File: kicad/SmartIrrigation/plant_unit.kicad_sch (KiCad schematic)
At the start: 10 parts, among them T1 RJ45 Connector

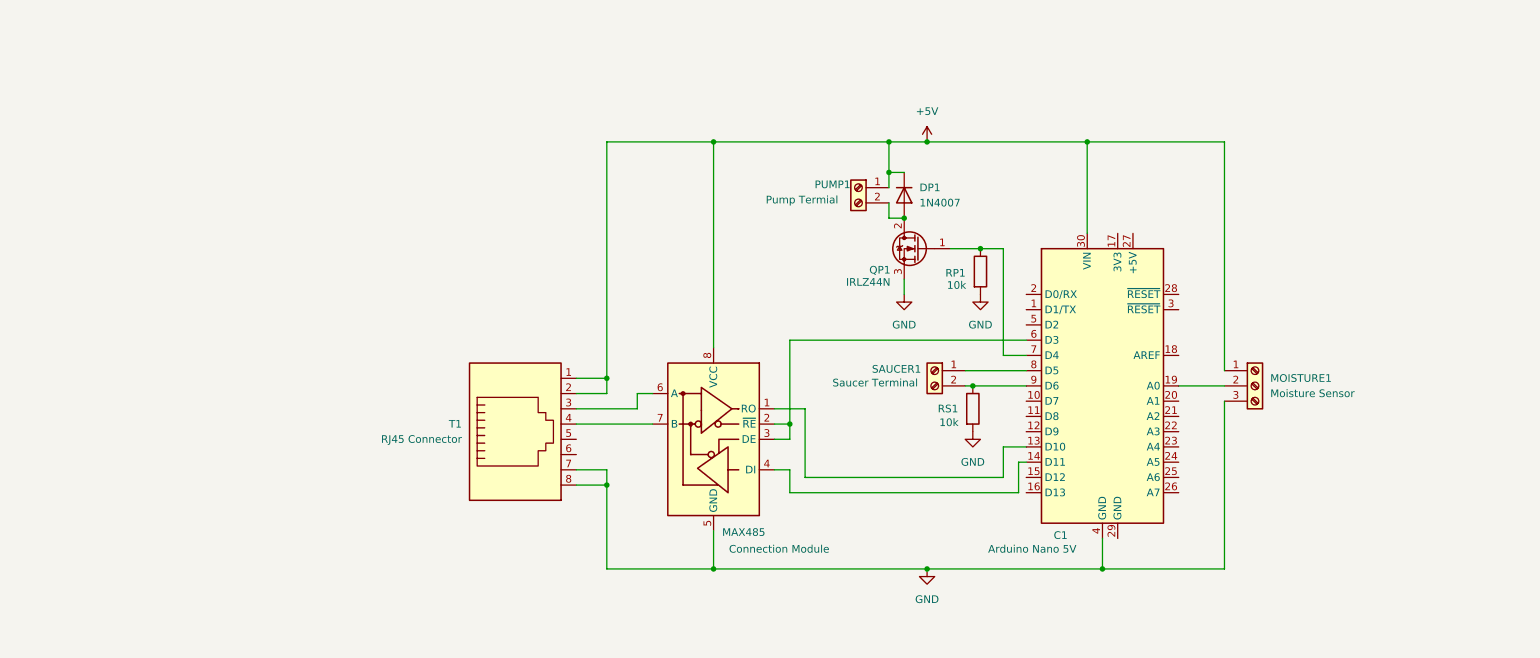
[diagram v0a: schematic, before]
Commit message: added schematics images
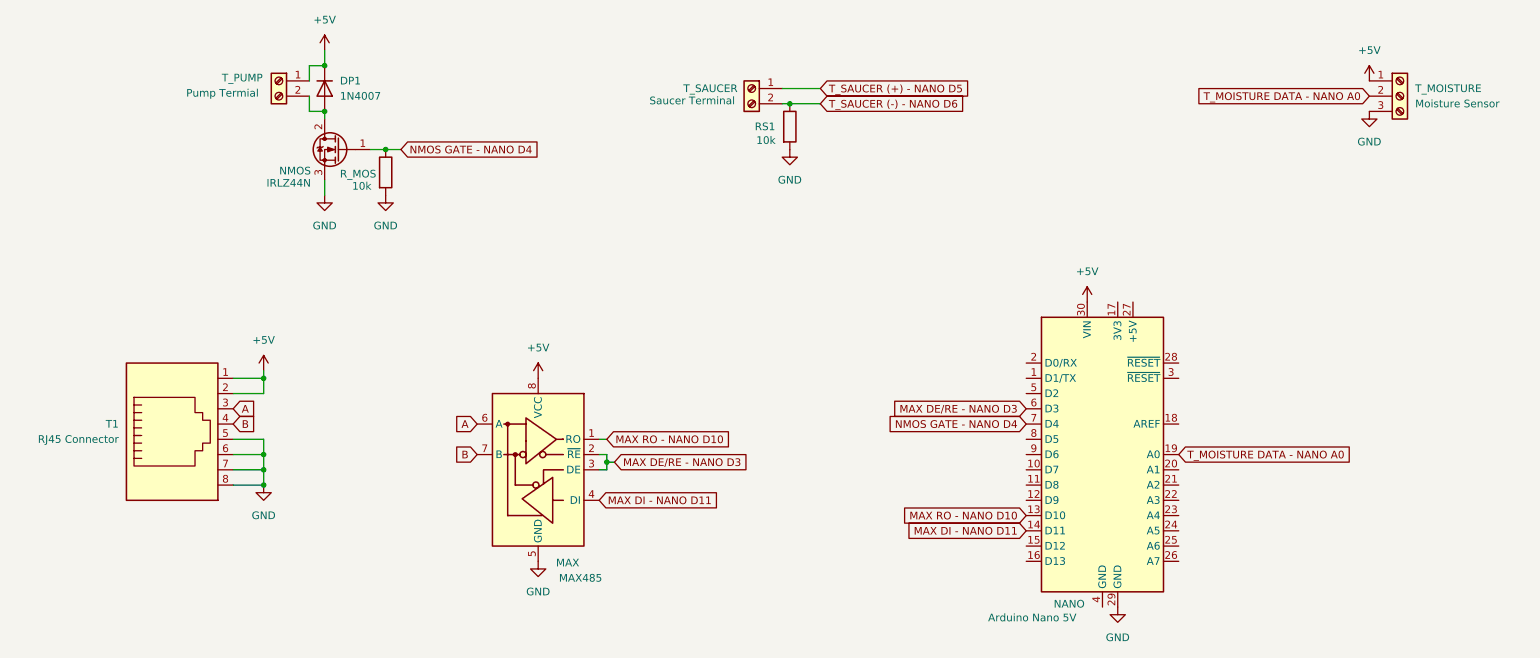
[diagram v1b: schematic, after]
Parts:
- MAX: renamed from MAX485; value Connection Module -> MAX485
- renumbered C1 to NANO, QP1 to NMOS, RP1 to R_MOS, MOISTURE1 to T_MOISTURE, PUMP1 to T_PUMP, SAUCER1 to T_SAUCER
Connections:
- net GND: now also NANO.29 (GND), T1.5, T1.6; no longer NANO.4 (GND)
- net NMOS GATE - NANO D4: now reaches NANO.7 (D4), NMOS.1 (G), R_MOS.1
- net A: now reaches MAX.6 (A), T1.3
- net B: now reaches MAX.7 (B), T1.4
- net MAX RO - NANO D10: now reaches MAX.1 (RO), NANO.13 (D10)
- net MAX DI - NANO D11: now reaches MAX.4 (DI), NANO.14 (D11)
- net T_MOISTURE DATA - NANO A0: now reaches NANO.19 (A0), T_MOISTURE.2 (Pin_2)
- net MAX DE/RE - NANO D3: now reaches MAX.2 (~{RE}), MAX.3 (DE), NANO.6 (D3)
- net at NANO.8 (D5): no longer T_SAUCER.1 (Pin_1)
- net T_SAUCER (-) -  NANO D6: now reaches RS1.1, T_SAUCER.2 (Pin_2)
- net T_SAUCER (-) -  NANO D6: no longer NANO.9 (D6)
- new net T_SAUCER (+) -  NANO D5: T_SAUCER.1 (Pin_1)
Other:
- moved on the sheet: DP1, MAX, NANO, NMOS, RS1, R_MOS, T1, T_MOISTURE, T_PUMP, T_SAUCER
